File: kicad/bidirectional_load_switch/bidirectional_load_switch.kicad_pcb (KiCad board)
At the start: 2 copper layers, 55 x 127 mm, 129 parts, among them J102 Conn_01x02_Socket, J103 Conn_01x09_Socket, J104 Conn_01x02_Socket, U101 LDL212PV33R, U201 SN74LVC1G17DCKR, U202 UCC23313DWYR, U203 SISS94DN-T1-GE3, U204 SISS94DN-T1-GE3, U301 SN74LVC1G17DCKR, U302 UCC23313DWYR, U303 SISS94DN-T1-GE3, U304 SISS94DN-T1-GE3, U401 SN74LVC1G17DCKR, U402 UCC23313DWYR, U403 SISS94DN-T1-GE3, U404 SISS94DN-T1-GE3, U501 SN74LVC1G17DCKR, U502 UCC23313DWYR, U503 SISS94DN-T1-GE3, U504 SISS94DN-T1-GE3, U601 SN74LVC1G17DCKR, U602 UCC23313DWYR, U603 SISS94DN-T1-GE3, U604 SISS94DN-T1-GE3, U701 SN74LVC1G17DCKR, U702 UCC23313DWYR, U703 SISS94DN-T1-GE3, U704 SISS94DN-T1-GE3, U801 SN74LVC1G17DCKR, U802 UCC23313DWYR, U803 SISS94DN-T1-GE3, U804 SISS94DN-T1-GE3, U901 SN74LVC1G17DCKR, U902 UCC23313DWYR, U903 SISS94DN-T1-GE3, U904 SISS94DN-T1-GE3

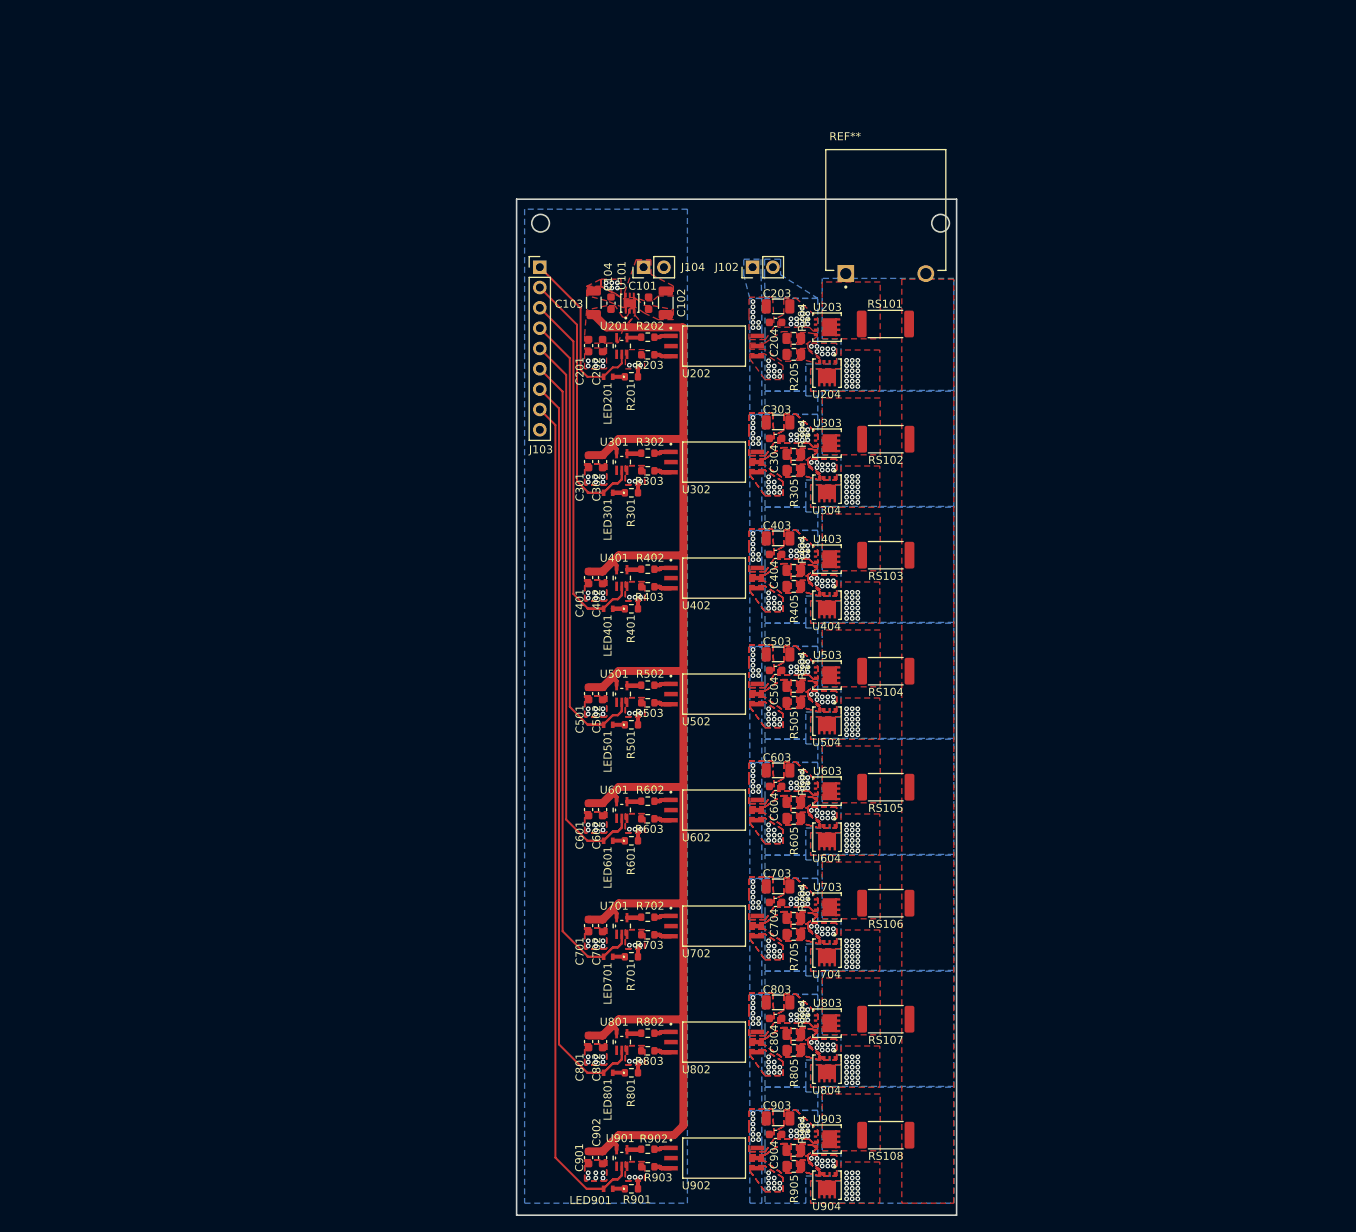
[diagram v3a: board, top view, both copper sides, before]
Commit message: i hate layouts
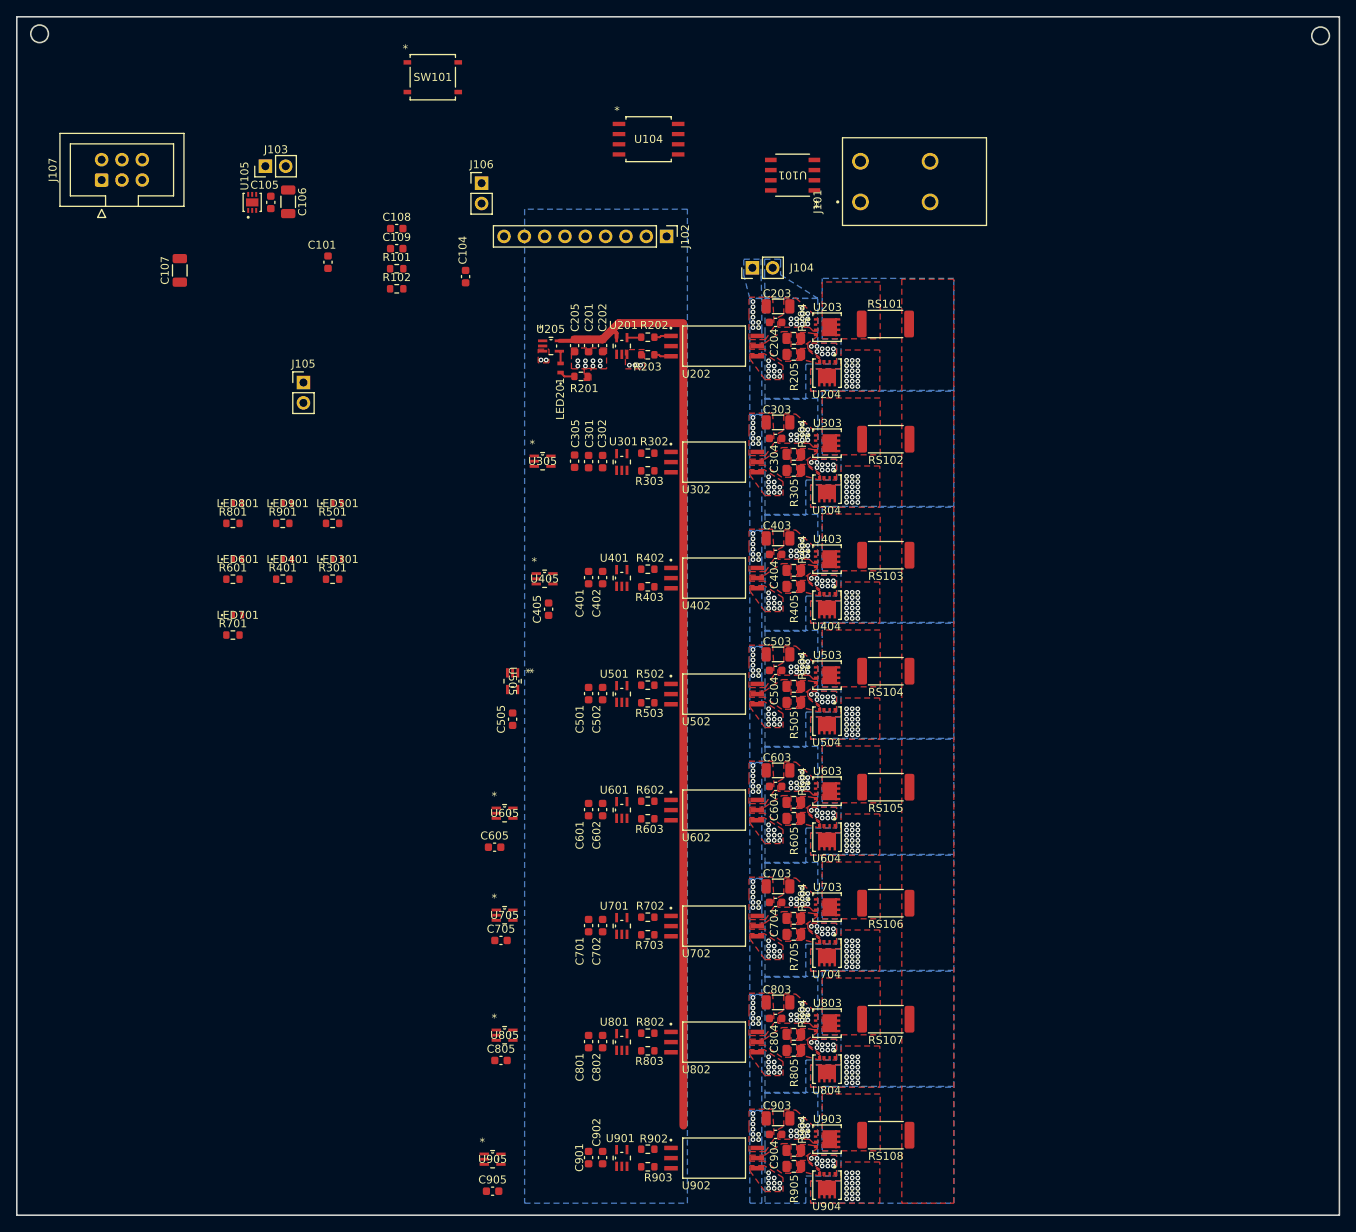
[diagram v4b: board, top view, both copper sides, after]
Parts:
- removed C102, C103: 10u, Capacitor_SMD:C_1206_3216Metric
- removed REF**: TE_282852-2, screw_terminal_282852-2:TE_282852-2
- added C105: 100n, Capacitor_SMD:C_0603_1608Metric, F.Cu at (59.3, 35.4)
- added C106: 10u, Capacitor_SMD:C_1206_3216Metric, F.Cu at (61.5, 35.3)
- added C107: 10u, Capacitor_SMD:C_1206_3216Metric, F.Cu at (47.9, 43.9)
- added C108: 100n, Capacitor_SMD:C_0603_1608Metric, F.Cu at (75.0, 38.7)
- added C109: 100n, Capacitor_SMD:C_0603_1608Metric, F.Cu at (75.0, 41.2)
- added C205: 100n, Capacitor_SMD:C_0603_1608Metric, F.Cu at (97.2, 53.3)
- added C305: 100n, Capacitor_SMD:C_0603_1608Metric, F.Cu at (97.2, 67.8)
- added C405: 100n, Capacitor_SMD:C_0603_1608Metric, F.Cu at (94.0, 86.2)
- added C505: 100n, Capacitor_SMD:C_0603_1608Metric, F.Cu at (89.5, 100.0)
- added C605: 100n, Capacitor_SMD:C_0603_1608Metric, F.Cu at (87.2, 116.0)
- added C705: 100n, Capacitor_SMD:C_0603_1608Metric, F.Cu at (88.0, 127.7)
- added C805: 100n, Capacitor_SMD:C_0603_1608Metric, F.Cu at (88.0, 142.7)
- added C905: 100n, Capacitor_SMD:C_0603_1608Metric, F.Cu at (87.0, 159.0)
- added J101: 1017503, spring_terminal_1017503:PHOENIX_1017503, F.Cu at (148.7, 38.3)
- added J105: Conn_01x02_Socket, Connector_PinHeader_2.54mm:PinHeader_1x02_P2.54mm_Vertical, F.Cu at (63.4, 57.9)
- added J106: Conn_01x02_Socket, Connector_PinHeader_2.54mm:PinHeader_1x02_P2.54mm_Vertical, F.Cu at (85.6, 33.0)
- added J107: AVR-ISP-6, Connector_IDC:IDC-Header_2x03_P2.54mm_Vertical, F.Cu at (38.1, 32.6)
- added R101: 10k, Resistor_SMD:R_0603_1608Metric, F.Cu at (75.0, 43.7)
- added R102: 10k, Resistor_SMD:R_0603_1608Metric, F.Cu at (75.0, 46.2)
- added SW101: PTS526 SK15 SMTR2 LFS, switch_switch_PTS526_SK15_SMTR2_LFS:SMT_FS, F.Cu at (79.5, 19.8)
- added U104: ATTINY85-20SU, mcu_ATTINY85_20SU:8S2_ATM, F.Cu at (106.5, 27.5)
- added U105: LDL212PV33R, ldo_LDL212PV33R:DFN_V33R_STM, F.Cu at (57.0, 35.4)
- added U205: SN74LVC1G08DCKR, and_gate_SN74LVC1G08DCKR:DCK5, F.Cu at (94.3, 53.4)
- added U305: SN74LVC1G08DCKR, and_gate_SN74LVC1G08DCKR:DCK5, F.Cu at (93.2, 67.8)
- added U405: SN74LVC1G08DCKR, and_gate_SN74LVC1G08DCKR:DCK5, F.Cu at (93.5, 82.5)
- added U505: SN74LVC1G08DCKR, and_gate_SN74LVC1G08DCKR:DCK5, F.Cu at (89.5, 95.2)
- added U605: SN74LVC1G08DCKR, and_gate_SN74LVC1G08DCKR:DCK5, F.Cu at (88.5, 111.8)
- added U705: SN74LVC1G08DCKR, and_gate_SN74LVC1G08DCKR:DCK5, F.Cu at (88.5, 124.5)
- added U805: SN74LVC1G08DCKR, and_gate_SN74LVC1G08DCKR:DCK5, F.Cu at (88.5, 139.5)
- added U905: SN74LVC1G08DCKR, and_gate_SN74LVC1G08DCKR:DCK5, F.Cu at (87.0, 155.0)
- J102: value Conn_01x02_Socket -> Conn_01x09_Socket; footprint Connector_PinHeader_2.54mm:PinHeader_1x02_P2.54mm_Vertical -> Connector_PinHeader_2.54mm:PinHeader_1x09_P2.54mm_Vertical
- J103: value Conn_01x09_Socket -> Conn_01x02_Socket; footprint Connector_PinHeader_2.54mm:PinHeader_1x09_P2.54mm_Vertical -> Connector_PinHeader_2.54mm:PinHeader_1x02_P2.54mm_Vertical
- U101: value LDL212PV33R -> TMCS1101A3BQDR; footprint ldo_LDL212PV33R:DFN_V33R_STM -> current_sensor_TMCS1101A3BQDR:SOIC8_D_TEX
- moved LED901 94.6 mm to (61.4, 73.0), turned to 0 degrees
- moved R901 93.9 mm to (60.8, 75.5)
- moved LED801 84.9 mm to (55.1, 73.0), turned to 0 degrees
- moved R801 84.8 mm to (54.5, 75.5)
- moved R701 64.0 mm to (54.5, 89.5)
- moved LED701 63.0 mm to (55.1, 87.0), turned to 0 degrees
- moved R601 59.6 mm to (54.5, 82.5)
- moved LED601 58.2 mm to (55.1, 80.0), turned to 0 degrees
- moved R501 45.0 mm to (67.0, 75.5)
- moved R401 43.7 mm to (60.8, 82.5)
- moved LED501 43.7 mm to (67.6, 73.0), turned to 0 degrees
- moved LED401 40.6 mm to (61.4, 80.0), turned to 0 degrees
- moved C101 40.4 mm to (66.4, 42.9)
- moved R301 38.9 mm to (67.0, 82.5)
- moved J103 36.5 mm to (58.6, 30.9), turned to 90 degrees
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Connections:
- net /Channel 1/ANODE renamed Net-(U202-ANODE)
- net /Channel 1/BOUT renamed Net-(U201-Y)
- net /Channel 1/VOUT renamed Net-(U202-VOUT)
- net /Channel 2/ANODE renamed Net-(U302-ANODE)
- net /Channel 2/BOUT renamed Net-(U301-Y)
- net /Channel 2/VOUT renamed Net-(U302-VOUT)
- net /Channel 3/ANODE renamed Net-(U402-ANODE)
- net /Channel 3/BOUT renamed Net-(U401-Y)
- net /Channel 3/VOUT renamed Net-(U402-VOUT)
- net /Channel 4/ANODE renamed Net-(U502-ANODE)
- net /Channel 4/BOUT renamed Net-(U501-Y)
- net /Channel 4/VOUT renamed Net-(U502-VOUT)
- net /Channel 5/ANODE renamed Net-(U602-ANODE)
- net /Channel 5/BOUT renamed Net-(U601-Y)
- net /Channel 5/VOUT renamed Net-(U602-VOUT)
- net /Channel 6/ANODE renamed Net-(U702-ANODE)
- net /Channel 6/BOUT renamed Net-(U701-Y)
- net /Channel 6/VOUT renamed Net-(U702-VOUT)
- net /Channel 7/ANODE renamed Net-(U802-ANODE)
- net /Channel 7/BOUT renamed Net-(U801-Y)
- net /Channel 7/VOUT renamed Net-(U802-VOUT)
- net /Channel 8/ANODE renamed Net-(U902-ANODE)
- net /Channel 8/BOUT renamed Net-(U901-Y)
- net /Channel 8/VOUT renamed Net-(U902-VOUT)
- C101 pad 1: 5V -> 3V3
- J102 pad 1: 15V_isolated -> PWM1_in
- J102 pad 2: GNDPWR -> PWM2_in
- J103 pad 1: /PWM1 -> GND
- J103 pad 2: /PWM2 -> 5V
- J104 pad 1: 5V -> 15V_isolated
- J104 pad 2: GND -> GNDPWR
- LED201 pad 2: /PWM1 -> Net-(U201-A)
- LED301 pad 2: /PWM2 -> Net-(U301-A)
- LED401 pad 2: /PWM3 -> Net-(U401-A)
- LED501 pad 2: /PWM4 -> Net-(U501-A)
- LED601 pad 2: /PWM5 -> Net-(U601-A)
- LED701 pad 2: /PWM6 -> Net-(U701-A)
- LED801 pad 2: /PWM7 -> Net-(U801-A)
- LED901 pad 2: /PWM8 -> Net-(U901-A)
- RS101 pad 1: /AC_in -> AC_post_sense
- RS102 pad 1: /AC_in -> AC_post_sense
- RS103 pad 1: /AC_in -> AC_post_sense
- RS104 pad 1: /AC_in -> AC_post_sense
- RS105 pad 1: /AC_in -> AC_post_sense
- RS106 pad 1: /AC_in -> AC_post_sense
- RS107 pad 1: /AC_in -> AC_post_sense
- RS108 pad 1: /AC_in -> AC_post_sense
- U101 pad 1: GND -> AC_post_sense
- U101 pad 2: 3V3 -> AC_post_sense
- U101 pad 3: 3V3 -> AC_in
- U101 pad 4: 5V -> AC_in
- U101 pad 5: unconnected-(U101-NC-Pad5) -> GND
- U101 pad 6: 5V -> unconnected-(U101-NC-Pad6)
- U101 pad 7: GND -> Net-(U101-VOUT)
- U201 pad 2: /PWM1 -> Net-(U201-A)
- U301 pad 2: /PWM2 -> Net-(U301-A)
- U401 pad 2: /PWM3 -> Net-(U401-A)
- U501 pad 2: /PWM4 -> Net-(U501-A)
- U601 pad 2: /PWM5 -> Net-(U601-A)
- U701 pad 2: /PWM6 -> Net-(U701-A)
- U801 pad 2: /PWM7 -> Net-(U801-A)
- U901 pad 2: /PWM8 -> Net-(U901-A)
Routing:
- net /PWM8: track 112.3 -> 0.00 mm
- net /PWM7: track 100.3 -> 0.00 mm
- net 3V3: track 209.1 -> 117.4 mm
- net /PWM6: track 88.3 -> 0.00 mm
- net /PWM5: track 76.3 -> 0.00 mm
- net /PWM4: track 64.4 -> 0.00 mm
- net /PWM3: track 52.3 -> 0.00 mm
- net /PWM2: track 40.4 -> 0.00 mm
- net /PWM1: track 22.3 -> 0.00 mm
- net GND: track 18.6 -> 0.00 mm, vias 78 -> 13
- net Net-(U902-CATHODE): track 4.31 -> 0.00 mm
- net Net-(U802-CATHODE): track 4.31 -> 0.00 mm
- net Net-(U502-CATHODE): track 4.31 -> 0.00 mm
- net Net-(U702-CATHODE): track 4.31 -> 0.00 mm
- net Net-(U602-CATHODE): track 4.31 -> 0.00 mm
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- added copper zone on F.Cu, net AC_post_sense
- removed copper zone on F.Cu, net /AC_in
- removed copper zone on F.Cu, net /Channel 3/VG2
- removed copper zone on F.Cu, net /Channel 6/VG1
- removed copper zone on F.Cu, net /Channel 6/VG2
- removed copper zone on F.Cu, net 3V3
- removed copper zone on F.Cu, net 5V
- removed copper zone on F.Cu, net Net-(U802-VOUT)
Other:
- board size 55 x 127 mm -> 165.3 x 149.8 mm

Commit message: :|
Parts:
- removed U105: LDL212PV33R, ldo_LDL212PV33R:DFN_V33R_STM
- added U102: TLV75733PDBVR, ldo_TLV75733PDBVR:DBV0005A_N, F.Cu at (102.8, 46.0)
- moved LED901 91.8 mm to (95.5, 158.3), turned to 90 degrees
- moved R901 91.7 mm to (98.0, 159.3)
- moved R801 81.8 mm to (98.0, 144.8)
- moved LED801 81.4 mm to (95.5, 143.7), turned to 90 degrees
- moved J107 64.2 mm to (101.8, 24.4), turned to -90 degrees
- moved R701 59.6 mm to (98.0, 130.2)
- moved LED701 58.3 mm to (95.5, 129.1), turned to 90 degrees
- moved C107 54.8 mm to (102.7, 42.7), turned to 0 degrees
- moved R601 54.6 mm to (98.0, 115.5)
- moved LED601 53.1 mm to (95.5, 114.5), turned to 90 degrees
- moved J102 51.4 mm to (75.8, 79.1), turned to 0 degrees
- moved J103 49.9 mm to (108.0, 37.9), turned to 0 degrees
- moved C106 48.2 mm to (108.5, 46.0), turned to -90 degrees
- moved C105 48.1 mm to (106.2, 46.0), turned to -90 degrees
- moved C101 45.5 mm to (111.7, 38.5)
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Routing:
- net 3V3: track 117.4 -> 141.5 mm
- net Net-(U702-CATHODE): track 0.00 -> 2.15 mm
- net Net-(U302-CATHODE): track 0.00 -> 2.15 mm
- net Net-(U602-CATHODE): track 0.00 -> 2.15 mm
- net Net-(U502-CATHODE): track 0.00 -> 2.15 mm
- net Net-(U402-CATHODE): track 0.00 -> 2.15 mm
- net Net-(U902-CATHODE): track 0.00 -> 2.15 mm
- net Net-(U802-CATHODE): track 0.00 -> 2.15 mm
- net Net-(U702-ANODE): track 0.00 -> 2.14 mm
- net Net-(U602-ANODE): track 0.00 -> 2.14 mm
- net Net-(U502-ANODE): track 0.00 -> 2.14 mm
- net Net-(U402-ANODE): track 0.00 -> 2.14 mm
- net Net-(U902-ANODE): track 0.00 -> 2.14 mm
- net Net-(U802-ANODE): track 0.00 -> 2.14 mm
- net Net-(U302-ANODE): track 0.00 -> 2.14 mm
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- added copper zone on F.Cu, net /Channel 3/VG2
- added copper zone on F.Cu, net /Channel 6/VG1
- added copper zone on F.Cu, net /Channel 6/VG2
- added copper zone on F.Cu, net AC_in
- added copper zone on F.Cu, net Net-(U802-VOUT)
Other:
- board size 165.3 x 149.8 mm -> 452.1 x 259 mm
